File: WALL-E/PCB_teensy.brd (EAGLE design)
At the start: 92.8 x 115.8 mm, 42 parts, among them U4 R-78E5.0-0.5

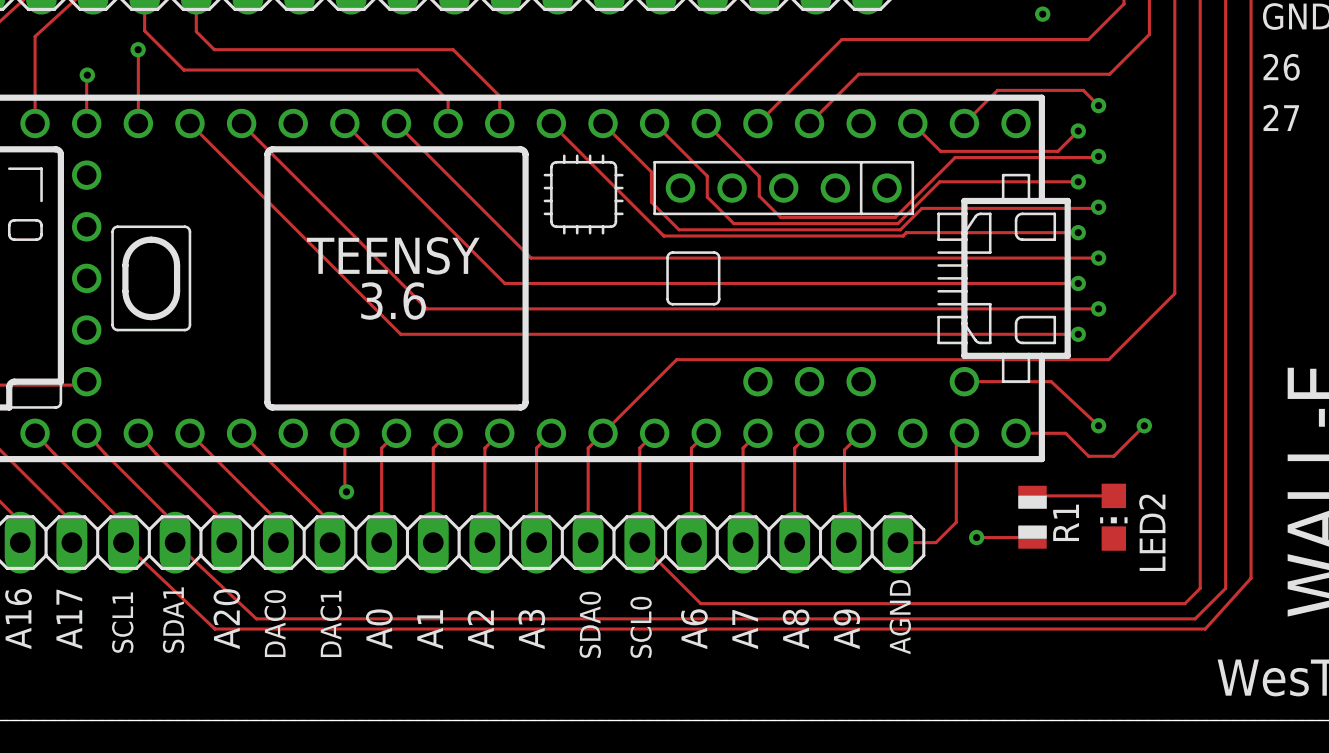
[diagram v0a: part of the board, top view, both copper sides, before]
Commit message: cleaned up each layer
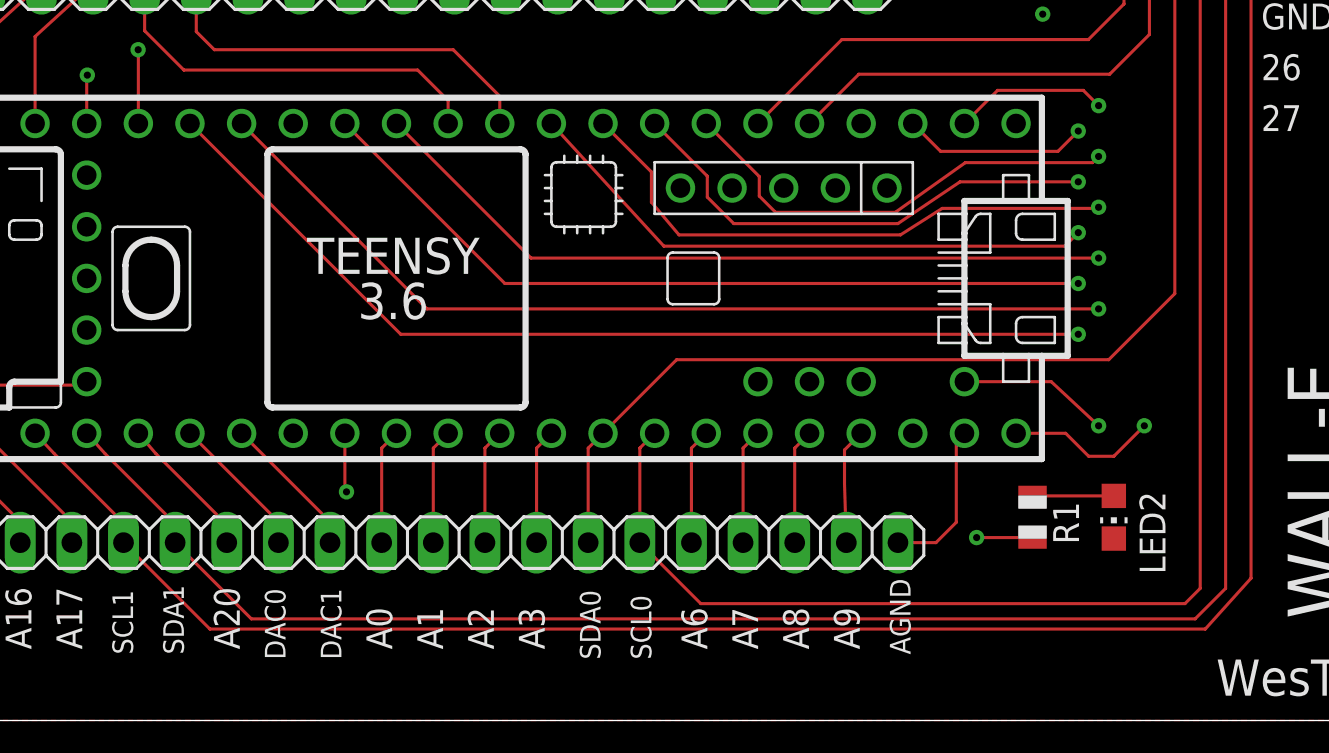
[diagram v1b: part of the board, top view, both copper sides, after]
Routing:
- net 8: track 90.0 -> 90.5 mm
- net 0/RX: track 94.4 -> 93.9 mm
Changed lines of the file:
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@@
 <contactref element="U$1" pad="0/RX"/>
 <contactref element="J1" pad="3"/>
-<wire x1="62.9" y1="29.37" x2="62.9" y2="28.85" width="0.1524" layer="1"/>
 <via x="69.5" y="30.25" extent="1-16" drill="0.35"/>
 <wire x1="74.98" y1="102.48" x2="86.75" y2="102.48" width="0.1524" layer="1"/>
@@
 <via x="69.5" y="27.75" extent="1-16" drill="0.35"/>
 <wire x1="50.2" y1="29.37" x2="52.8075" y2="26.7625" width="0.1524" layer="1"/>
-<wire x1="52.8075" y1="26.7625" x2="52.8075" y2="25.80045625" width="0.1524" layer="1"/>
-<wire x1="52.8075" y1="25.80045625" x2="53.85795625" y2="24.75" width="0.1524" layer="1"/>
-<wire x1="53.85795625" y1="24.75" x2="59.5" y2="24.75" width="0.1524" layer="1"/>
-<wire x1="59.5" y1="24.75" x2="62.4452" y2="27.6952" width="0.1524" layer="1"/>
-<wire x1="69.4452" y1="27.6952" x2="69.5" y2="27.75" width="0.1524" layer="1"/>
-<wire x1="62.4452" y1="27.6952" x2="69.4452" y2="27.6952" width="0.1524" layer="1"/>
+<wire x1="52.8075" y1="25.80045625" x2="52.8075" y2="26.7625" width="0.1524" layer="1"/>
+<wire x1="59.5" y1="25" x2="62.9452" y2="27.4452" width="0.1524" layer="1"/>
 <wire x1="69.5" y1="27.75" x2="73.25" y2="31.5" width="0.1524" layer="15"/>
 <wire x1="73.25" y1="31.5" x2="73.25" y2="84.25" width="0.1524" layer="15"/>
@@
 <wire x1="73.25" y1="84.25" x2="77.48" y2="88.48" width="0.1524" layer="1"/>
 <wire x1="77.48" y1="88.48" x2="86.75" y2="88.48" width="0.1524" layer="1"/>
+<wire x1="53.60795625" y1="25" x2="52.8075" y2="25.80045625" width="0.1524" layer="1"/>
+<wire x1="59.5" y1="25" x2="53.60795625" y2="25" width="0.1524" layer="1"/>
+<wire x1="69.1952" y1="27.4452" x2="69.5" y2="27.75" width="0.1524" layer="1"/>
+<wire x1="62.9452" y1="27.4452" x2="69.1952" y2="27.4452" width="0.1524" layer="1"/>
 </signal>
 <signal name="6">
@@
 <via x="68.5" y="26.5" extent="1-16" drill="0.35"/>
 <wire x1="50.25" y1="25.75" x2="51.5548" y2="24.4452" width="0.1524" layer="1"/>
-<wire x1="61.68105625" y1="26.5" x2="68.5" y2="26.5" width="0.1524" layer="1"/>
-<wire x1="59.62625625" y1="24.4452" x2="61.68105625" y2="26.5" width="0.1524" layer="1"/>
+<wire x1="62.68105625" y1="26.5" x2="68.5" y2="26.5" width="0.1524" layer="1"/>
+<wire x1="59.62625625" y1="24.4452" x2="62.68105625" y2="26.5" width="0.1524" layer="1"/>
 <wire x1="51.5548" y1="24.4452" x2="59.62625625" y2="24.4452" width="0.1524" layer="1"/>
 <wire x1="68.5" y1="26.5" x2="69.75" y2="26.5" width="0.1524" layer="15"/>
@@
 <wire x1="45.12" y1="29.37" x2="47.5" y2="26.99" width="0.1524" layer="1"/>
 <wire x1="47.5" y1="26.99" x2="47.5" y2="25.5" width="0.1524" layer="1"/>
-<wire x1="47.5" y1="25.5" x2="48.8596" y2="24.1404" width="0.1524" layer="1"/>
-<wire x1="48.8596" y1="24.1404" x2="59.7525125" y2="24.1404" width="0.1524" layer="1"/>
-<wire x1="59.7525125" y1="24.1404" x2="60.80605625" y2="25.19394375" width="0.1524" layer="1"/>
-<wire x1="60.80605625" y1="25.19394375" x2="69.44394375" y2="25.19394375" width="0.1524" layer="1"/>
+<wire x1="47.5" y1="25.5" x2="48.8596" y2="23.8904" width="0.1524" layer="1"/>
+<wire x1="48.8596" y1="23.8904" x2="59.7525125" y2="23.8904" width="0.1524" layer="1"/>
+<wire x1="59.7525125" y1="23.8904" x2="61.80605625" y2="25.19394375" width="0.1524" layer="1"/>
+<wire x1="61.80605625" y1="25.19394375" x2="69.44394375" y2="25.19394375" width="0.1524" layer="1"/>
 <wire x1="69.44394375" y1="25.19394375" x2="69.5" y2="25.25" width="0.1524" layer="1"/>
 <via x="69.5" y="25.25" extent="1-16" drill="0.35"/>
@@
 <contactref element="J3" pad="4"/>
 <via x="68.5" y="24" extent="1-16" drill="0.35"/>
-<wire x1="59.87876875" y1="23.8356" x2="60.04316875" y2="24" width="0.1524" layer="1"/>
-<wire x1="60.04316875" y1="24" x2="68.5" y2="24" width="0.1524" layer="1"/>
-<wire x1="42.58" y1="29.37" x2="48.1144" y2="23.8356" width="0.1524" layer="1"/>
-<wire x1="48.1144" y1="23.8356" x2="59.87876875" y2="23.8356" width="0.1524" layer="1"/>
+<wire x1="48.1144" y1="23.3356" x2="42.58" y2="29.37" width="0.1524" layer="1"/>
 <wire x1="68.5" y1="24" x2="70" y2="24" width="0.1524" layer="15"/>
 <wire x1="70" y1="24" x2="76.25" y2="30.25" width="0.1524" layer="15"/>
@@
 <wire x1="76.25" y1="70.5" x2="77.69" y2="71.94" width="0.1524" layer="1"/>
 <wire x1="77.69" y1="71.94" x2="86.75" y2="71.94" width="0.1524" layer="1"/>
+<wire x1="68.5" y1="24" x2="67.8356" y2="23.3356" width="0.1524" layer="1"/>
+<wire x1="67.8356" y1="23.3356" x2="48.1144" y2="23.3356" width="0.1524" layer="1"/>
 </signal>
 <signal name="24">
@@
 <via x="66.75" y="37" extent="1-16" drill="0.35"/>
 <wire x1="66.75" y1="37" x2="76.75" y2="37" width="0.1524" layer="2"/>
-<wire x1="76.75" y1="37" x2="77" y2="37" width="0.1524" layer="2"/>
 <via x="81.75" y="26.25" extent="1-16" drill="0.35"/>
 <wire x1="81.75" y1="26.25" x2="81.77" y2="26.23" width="0.1524" layer="1"/>
@@
 <wire x1="21.53" y1="9.72" x2="21.53" y2="8.75" width="0.1524" layer="1"/>
 <wire x1="18.12" y1="13.13" x2="21.53" y2="9.72" width="0.1524" layer="1"/>
-<wire x1="21.53" y1="8.75" x2="26.03" y2="4.5" width="0.1524" layer="1"/>
-<wire x1="26.03" y1="4.5" x2="74.75" y2="4.5" width="0.1524" layer="1"/>
+<wire x1="21.53" y1="8.75" x2="25.78" y2="4.5" width="0.1524" layer="1"/>
+<wire x1="25.78" y1="4.5" x2="74.75" y2="4.5" width="0.1524" layer="1"/>
 <wire x1="74.75" y1="4.5" x2="77" y2="7" width="0.1524" layer="1"/>
 <wire x1="77" y1="7" x2="77" y2="39.5" width="0.1524" layer="1"/>
@@
 <wire x1="24.07" y1="9.68" x2="24.07" y2="8.75" width="0.1524" layer="1"/>
 <wire x1="20.62" y1="13.13" x2="24.07" y2="9.68" width="0.1524" layer="1"/>
-<wire x1="24.07" y1="8.75" x2="28.07" y2="5" width="0.1524" layer="1"/>
-<wire x1="28.07" y1="5" x2="74.25" y2="5" width="0.1524" layer="1"/>
+<wire x1="24.07" y1="8.75" x2="27.82" y2="5" width="0.1524" layer="1"/>
+<wire x1="27.82" y1="5" x2="74.25" y2="5" width="0.1524" layer="1"/>
 <wire x1="74.25" y1="5" x2="75.75" y2="6.5" width="0.1524" layer="1"/>
 <wire x1="75.75" y1="6.5" x2="75.75" y2="39.5" width="0.1524" layer="1"/>
